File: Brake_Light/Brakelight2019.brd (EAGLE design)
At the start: 59.9 x 39.8 mm, 49 parts

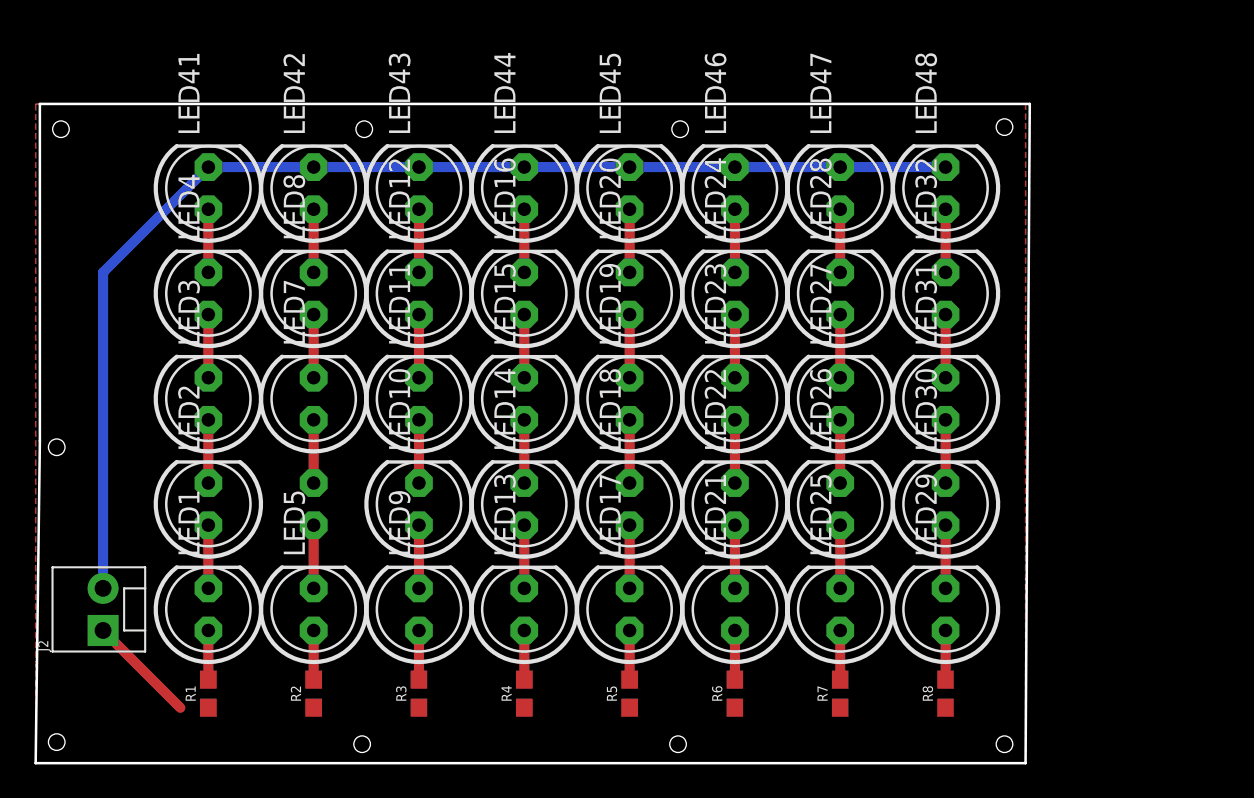
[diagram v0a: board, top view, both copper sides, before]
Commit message: Add files via upload
Brakelight is done!
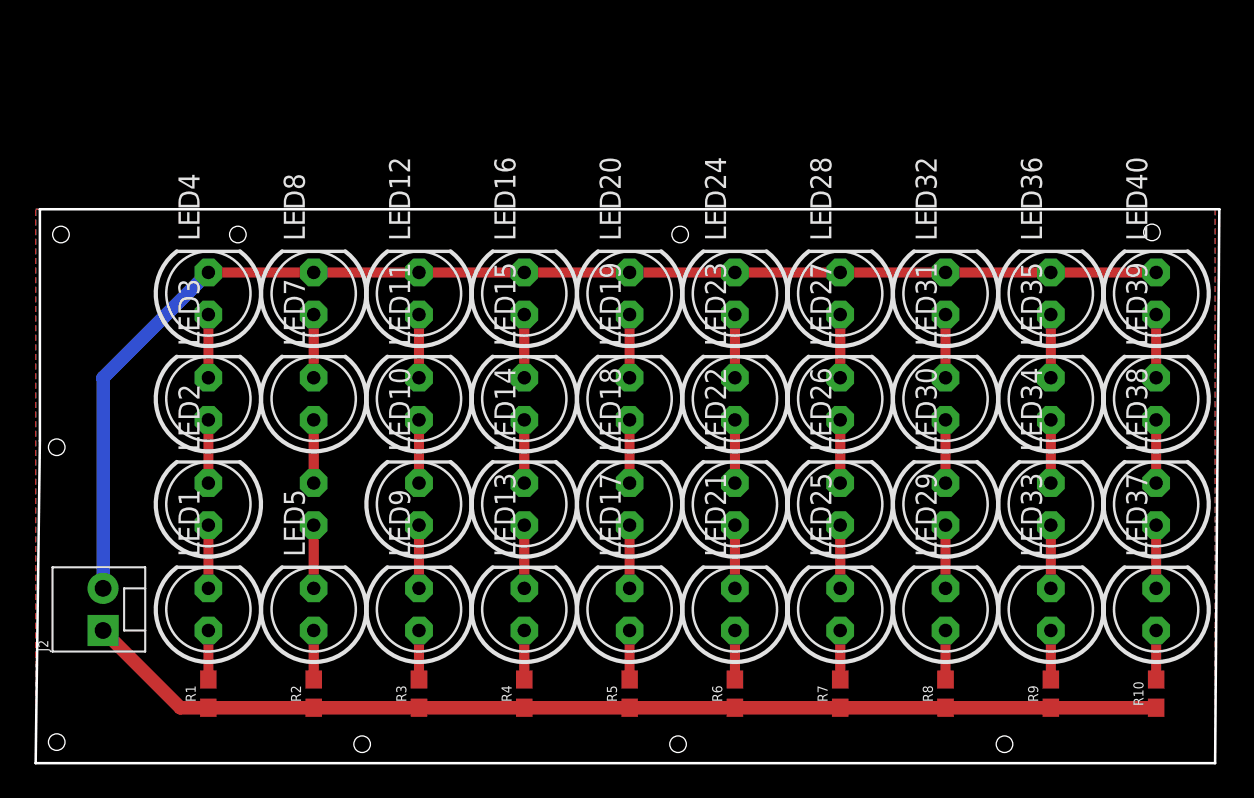
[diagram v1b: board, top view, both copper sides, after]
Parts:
- removed LED41, LED42, LED43, LED44, LED45, LED46, LED47, LED48: (no value), adafruit:LED5MM
- added LED33, LED34, LED35, LED36, LED37, LED38, LED39, LED40: (no value), adafruit:LED5MM
- added R10, R9: 68OHM-0603-1/10W-1%, SparkFun-Resistors:0603
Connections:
- removed net N$41: LED4.K, LED41.A
- removed net N$42: LED42.A, LED8.K
- removed net N$43: LED12.K, LED43.A
- removed net N$44: LED16.K, LED44.A
- removed net N$45: LED20.K, LED45.A
- removed net N$46: LED24.K, LED46.A
- removed net N$47: LED28.K, LED47.A
- removed net N$48: LED32.K, LED48.A
- new net N$33: LED33.A, R9.2
- new net N$34: LED33.K, LED34.A
- new net N$35: LED34.K, LED35.A
- new net N$36: LED35.K, LED36.A
- new net N$37: LED37.A, R10.2
- new net N$38: LED37.K, LED38.A
- new net N$39: LED38.K, LED39.A
- new net N$40: LED39.K, LED40.A
- net 12V: now also R10.1, R9.1
- net GND: now also LED12.K, LED16.K, LED20.K, LED24.K, LED28.K, LED32.K, LED36.K, LED4.K, LED40.K, LED8.K; no longer LED41.K, LED42.K, LED43.K, LED44.K, LED45.K, LED46.K, LED47.K, LED48.K
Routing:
- net 12V: track 6.59 -> 65.4 mm
- net GND: track 72.5 -> 78.8 mm
- net N$48: track 3.81 -> 0.00 mm
- net N$47: track 3.81 -> 0.00 mm
- net N$46: track 3.81 -> 0.00 mm
- net N$45: track 3.81 -> 0.00 mm
- net N$44: track 3.81 -> 0.00 mm
- net N$43: track 3.81 -> 0.00 mm
- net N$42: track 3.81 -> 0.00 mm
- net N$41: track 3.81 -> 0.00 mm
- net N$40: track 0.00 -> 3.81 mm
- net N$36: track 0.00 -> 3.81 mm
- net N$38: track 0.00 -> 3.81 mm
- net N$34: track 0.00 -> 3.81 mm
- net N$39: track 0.00 -> 3.81 mm
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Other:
- board size 59.9 x 39.8 mm -> 71.4 x 33.4 mm
